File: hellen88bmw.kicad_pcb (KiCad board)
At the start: 2 copper layers, 160 x 118 mm, 116 parts, among them J1 Conn_01x05, J10 Conn_01x12, J11 Conn_01x12, J12 Conn_01x12, J13 Conn_01x12, J2 Conn_01x05, J3 Micro_SD_Card, J4 Conn_01x05, J5 Conn_01x12, J6 Conn_01x12, J7 Conn_01x12, J8 Conn_01x12, J9 Conn_01x12, Q1 NGD8201AN, Q2 NGD8201AN, Q3 NGD8201AN, Q4 NGD8201AN, Q5 NGD8201AN, Q6 NGD8201AN, U1 MPXA6115A, U2 molex_48pin_MRE, U3 MPX4_MAP

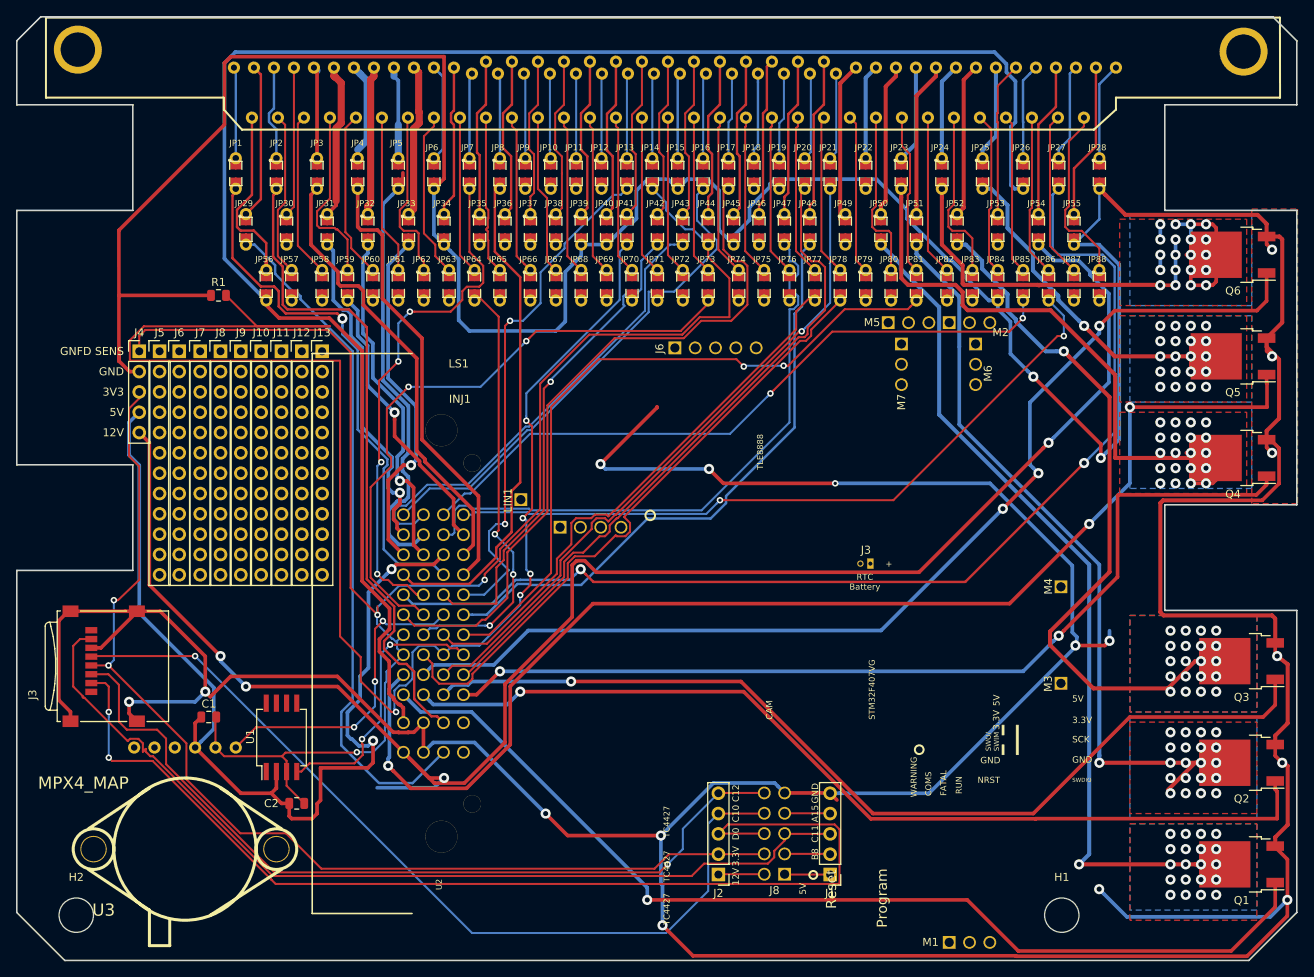
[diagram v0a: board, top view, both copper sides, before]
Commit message: Up 88bmw update
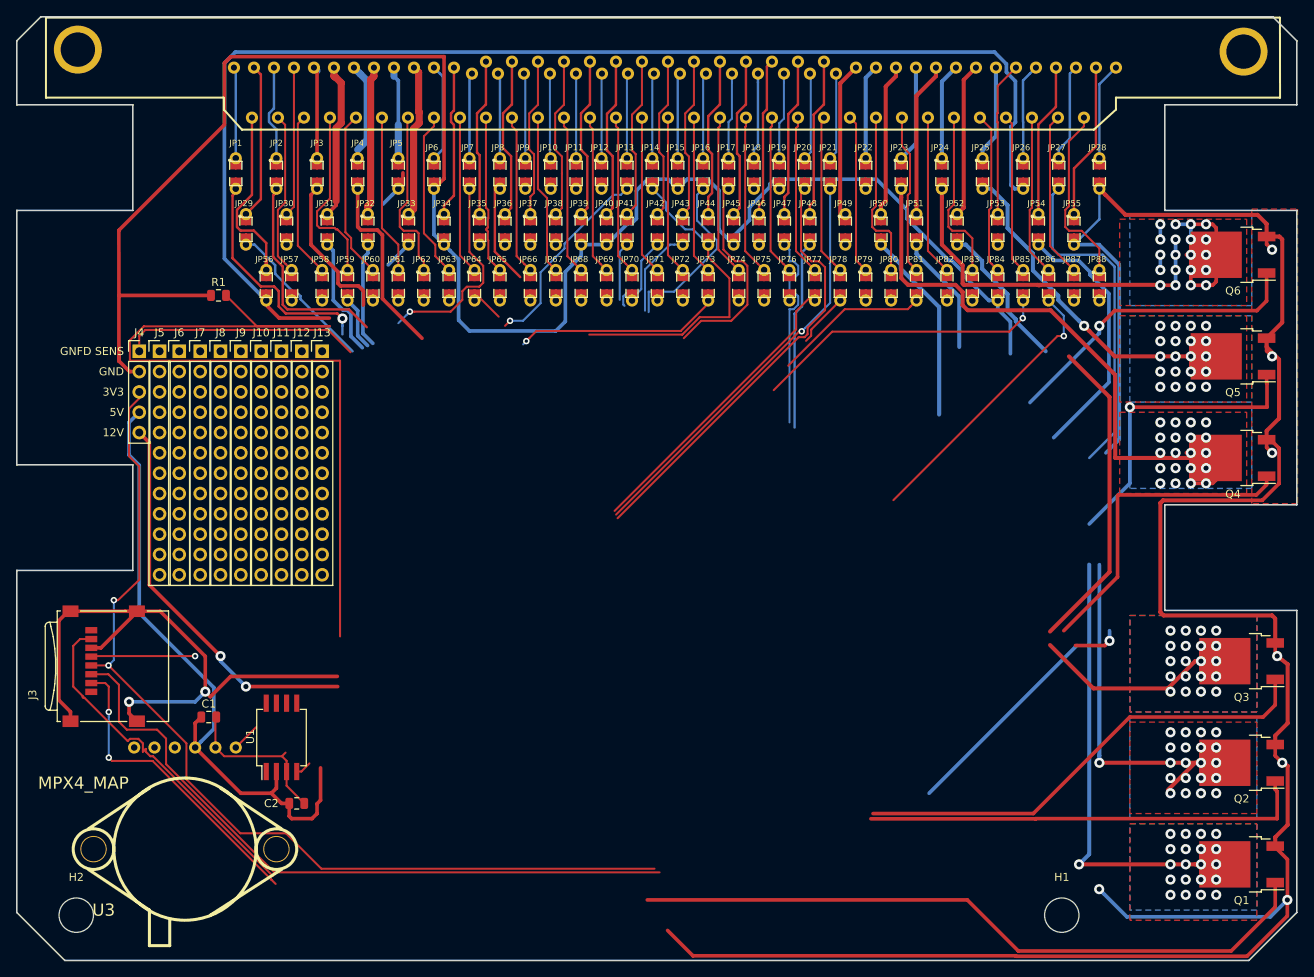
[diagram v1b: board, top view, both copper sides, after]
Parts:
- removed J1, J2: Conn_01x05, Connector_PinHeader_2.54mm:PinHeader_1x05_P2.54mm_Vertical
- removed U2: molex_48pin_MRE, rusefi_lib:Molex_48_MRE_with-extras
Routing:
- net GND: track 842.1 -> 635.7 mm, vias 19 -> 10
- net /12_MAIN_RELAY: track 218.1 -> 81.2 mm, vias 4 -> 2
- net /GND_SENS: track 209.6 -> 89.8 mm, vias 3 -> 0
- net /GP6: track 156.9 -> 37.9 mm, vias 3 -> 1
- net /J806_PB9: track 137.6 -> 38.7 mm
- net /J808_PC10: track 109.6 -> 13.0 mm
- net /GP5: track 135.4 -> 38.9 mm, vias 3 -> 1
- net /MAIN_RELAY: track 136.8 -> 41.7 mm, vias 2 -> 0
- net /MAF_AV4: track 194.3 -> 110.8 mm, vias 5 -> 0
- net /IGN_4: track 118.3 -> 39.9 mm, vias 2 -> 0
- net /J805_PC11: track 116.7 -> 43.9 mm
- net /CLT_AT1: track 78.6 -> 6.82 mm
- net /NEUTRAL_IN_AT3: track 86.9 -> 19.4 mm, vias 2 -> 0
- net /IDLE_LS2: track 85.9 -> 19.7 mm
- net /IGN_2: track 119.3 -> 55.6 mm, vias 1 -> 0
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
